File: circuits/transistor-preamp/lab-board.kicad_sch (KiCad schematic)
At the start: 32 parts, among them J1 Conn_01x02, J2 Conn_01x02, J3 Conn_01x02, Q1 2N3904

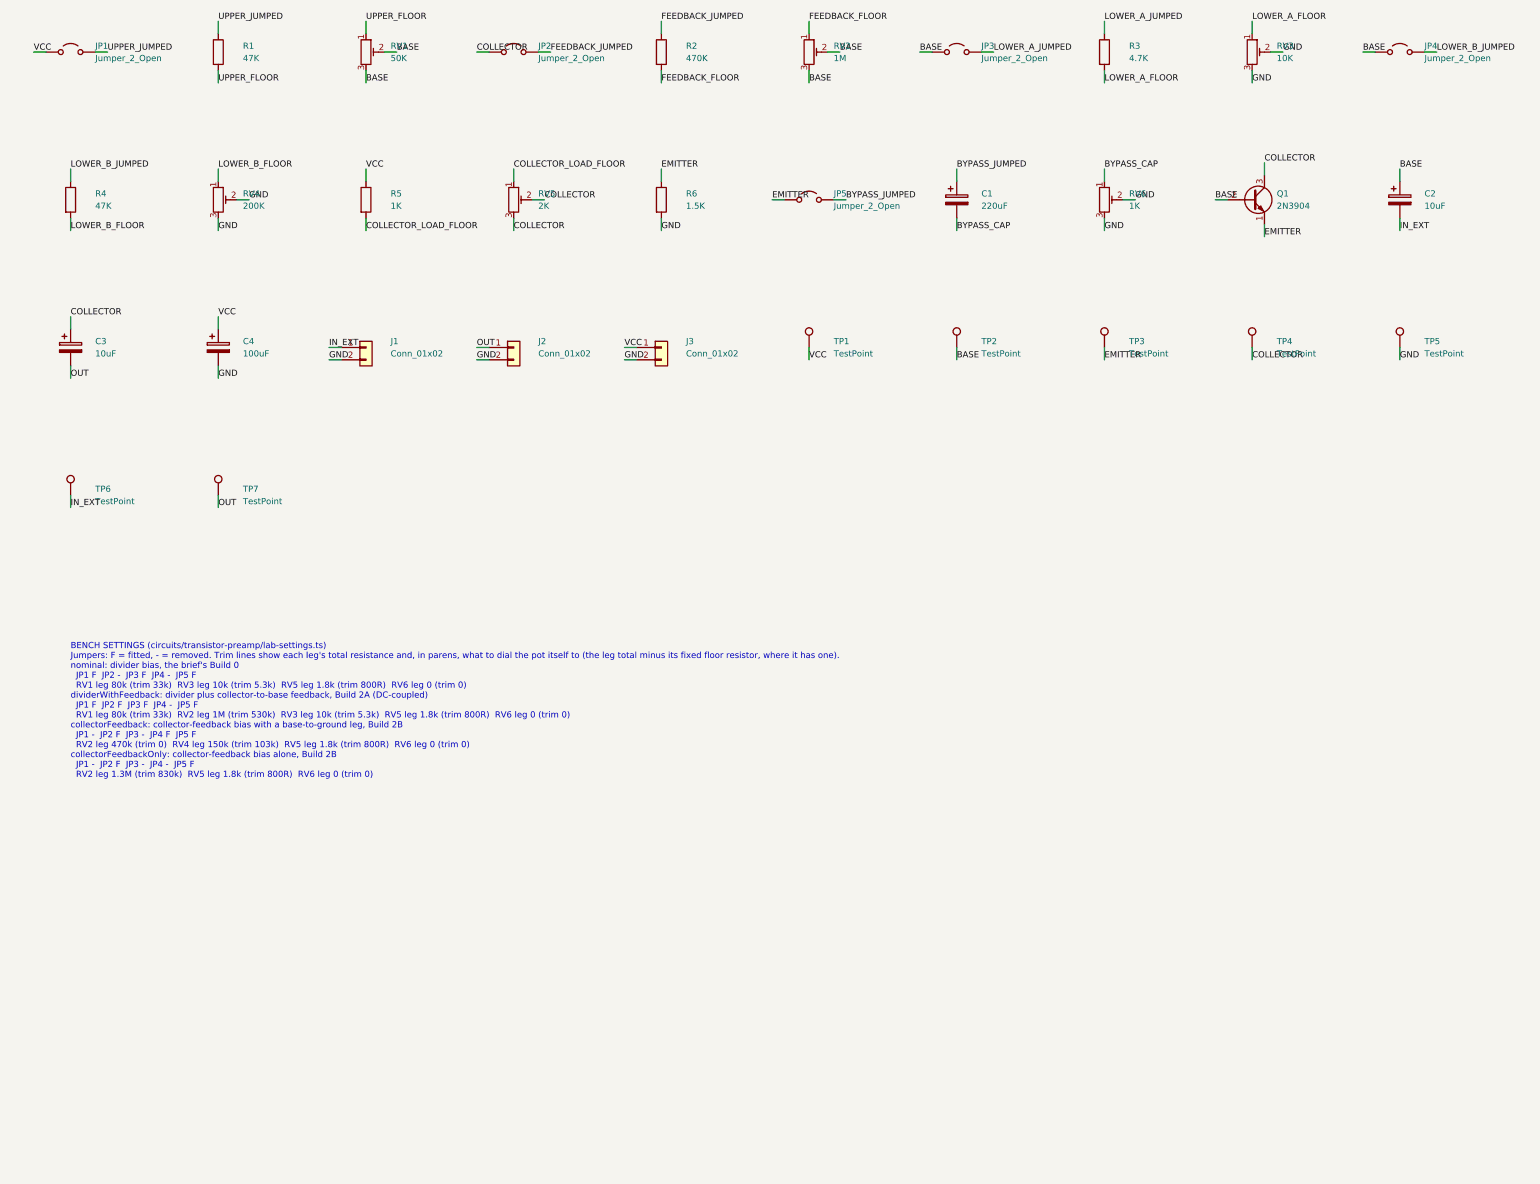
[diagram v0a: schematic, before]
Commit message: layout
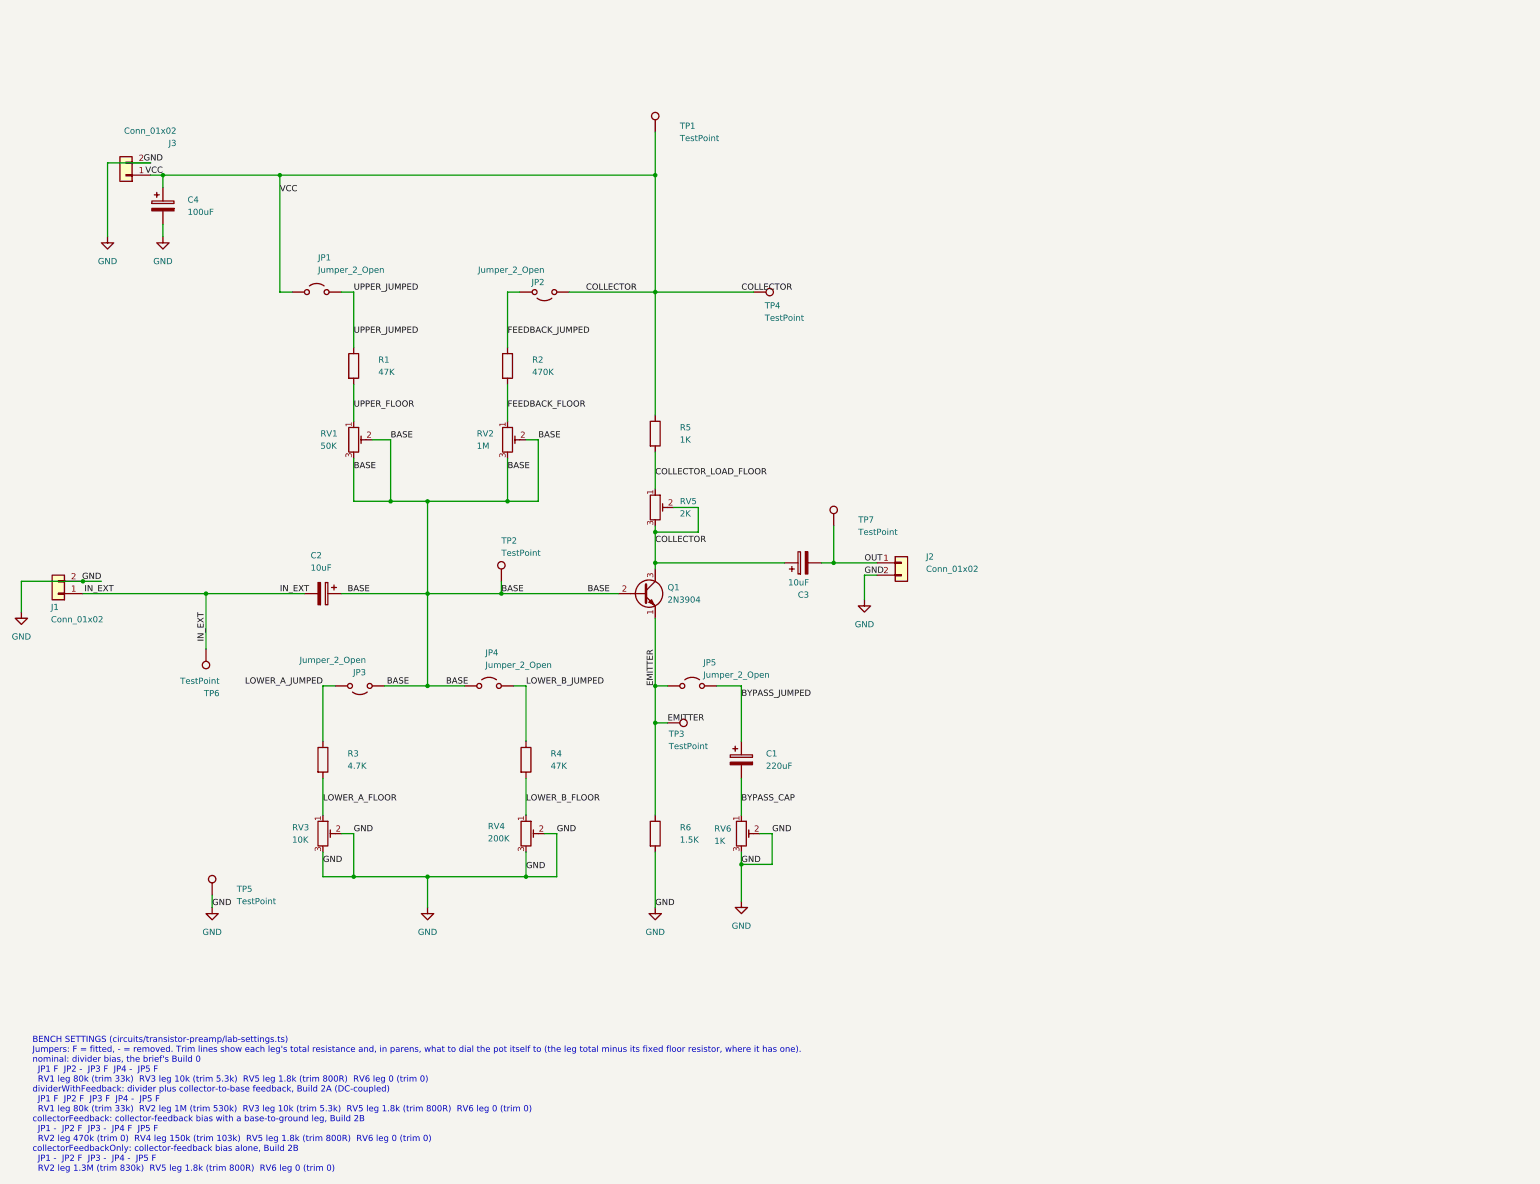
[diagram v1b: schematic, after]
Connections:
- net VCC is gone; now on net COLLECTOR: C4.1, J3.1 (Pin_1), JP1.1 (A), R5.1, TP1.1
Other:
- moved on the sheet: C1, C2, C3, C4, J1, J2, J3, JP1, JP2, JP3, JP4, JP5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

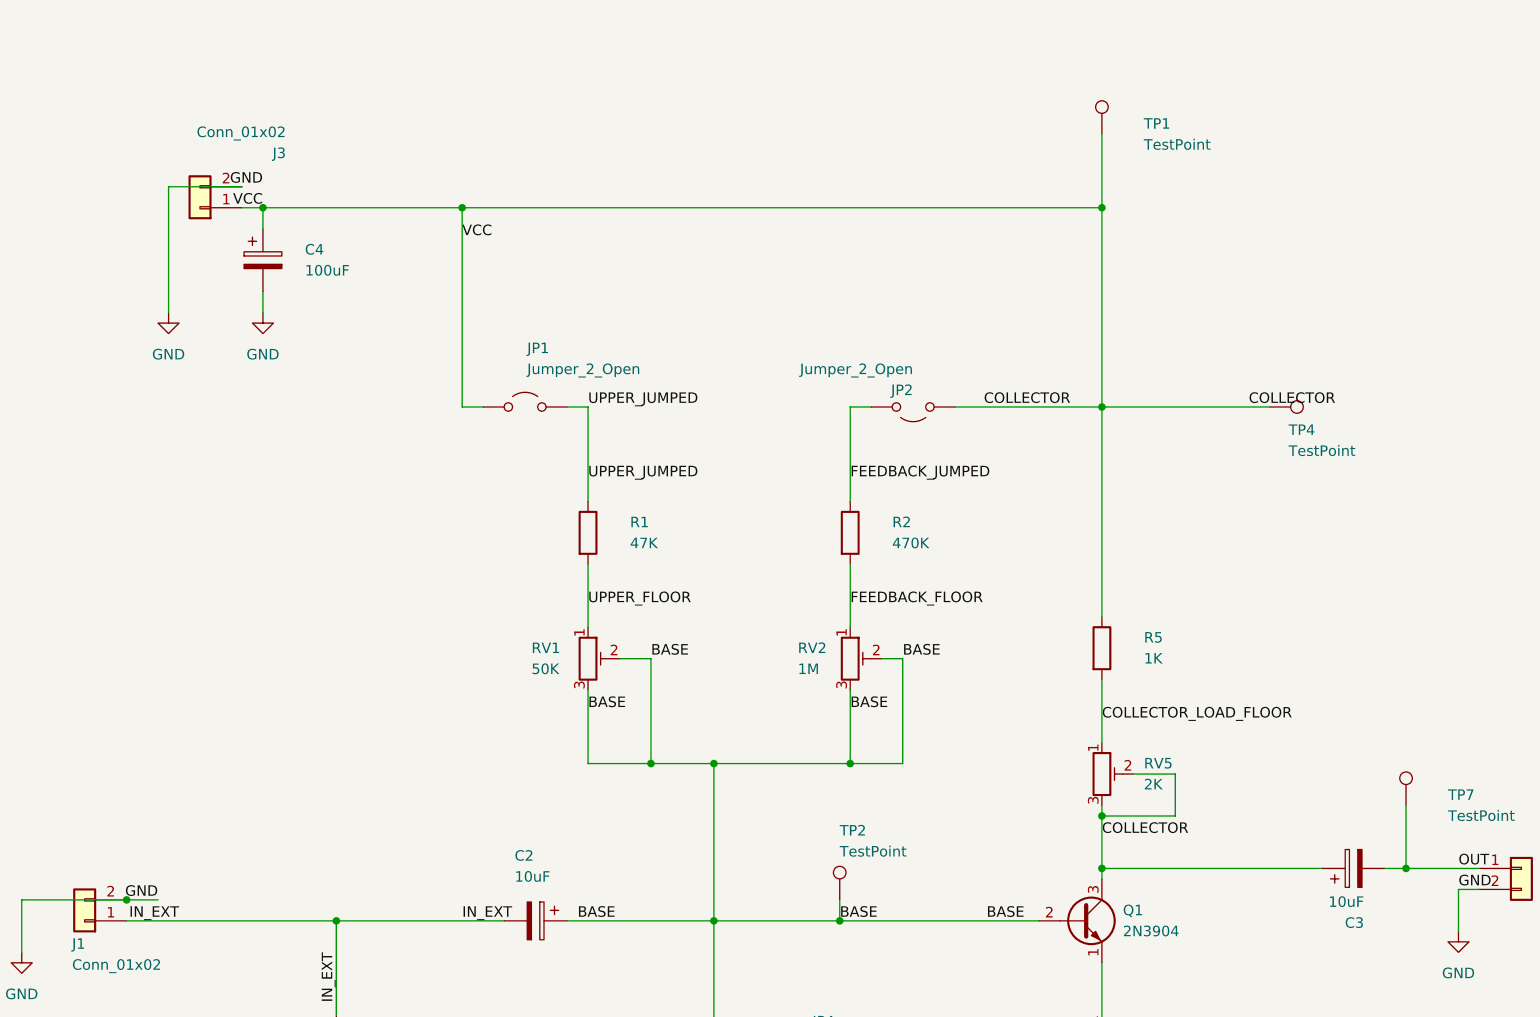
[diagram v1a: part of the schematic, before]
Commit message: repair
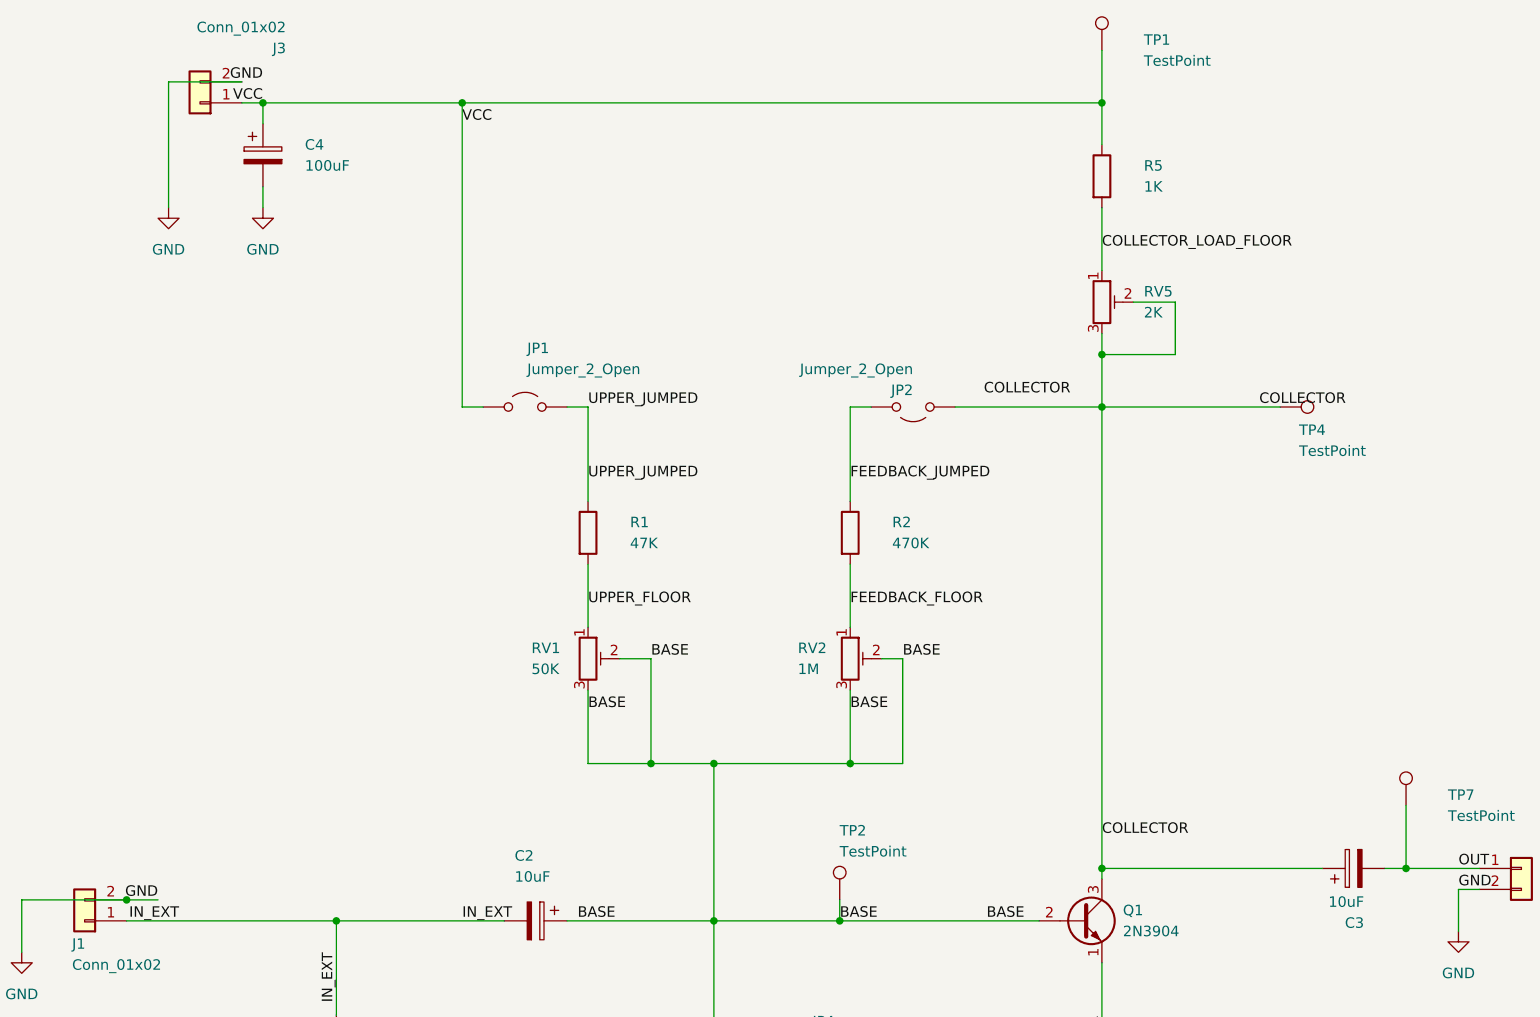
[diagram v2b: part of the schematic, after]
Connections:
- net COLLECTOR: no longer C4.1, J3.1 (Pin_1), JP1.1 (A), R5.1, TP1.1
- new net VCC: C4.1, J3.1 (Pin_1), JP1.1 (A), R5.1, TP1.1
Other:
- moved on the sheet: C4, J3, R5, RV5, TP1, TP4
